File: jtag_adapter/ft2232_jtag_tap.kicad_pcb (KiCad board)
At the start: 2 copper layers, 50 x 30 mm, 50 parts, among them J1 USB_C_Receptacle_USB2.0, J2 Conn_ARM_JTAG_SWD_20, U1 93AA56BT-I/OT, U2 FT232HL, Y1 Crystal_GND24

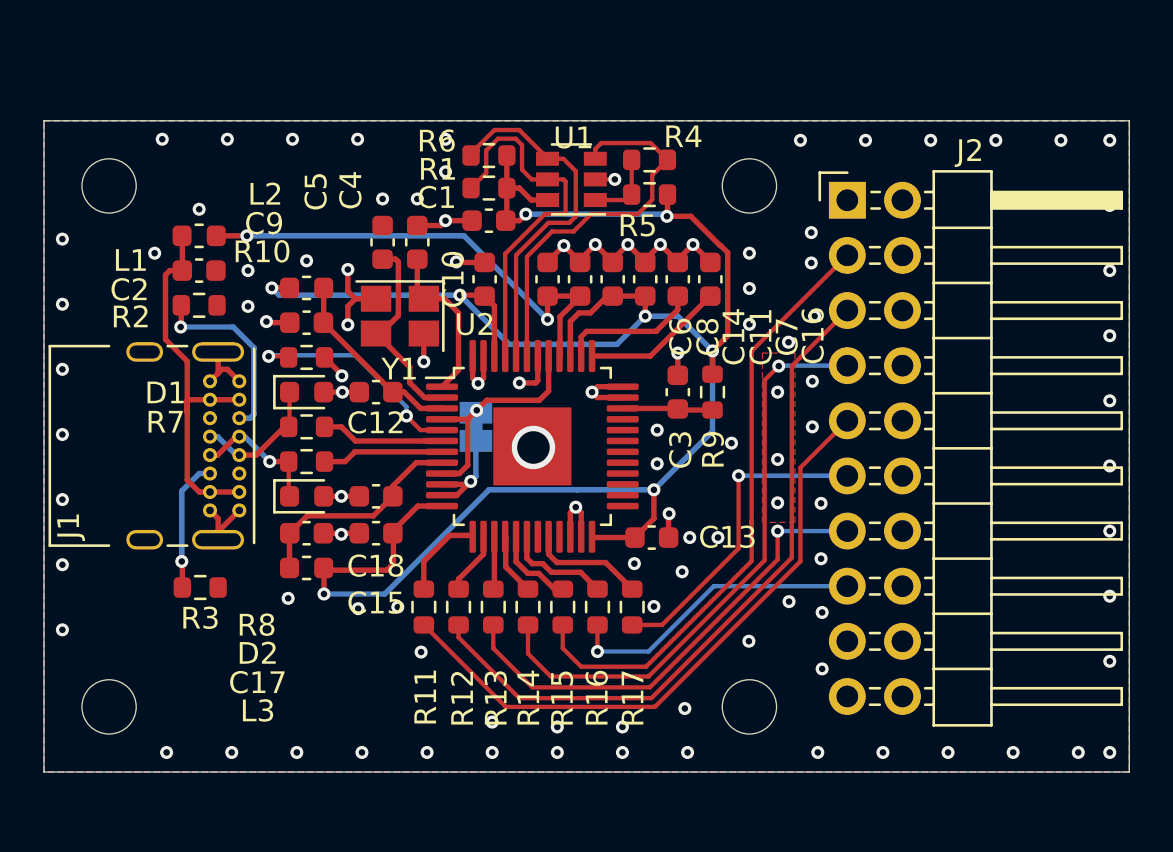
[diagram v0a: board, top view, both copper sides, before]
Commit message: v0.2に改修
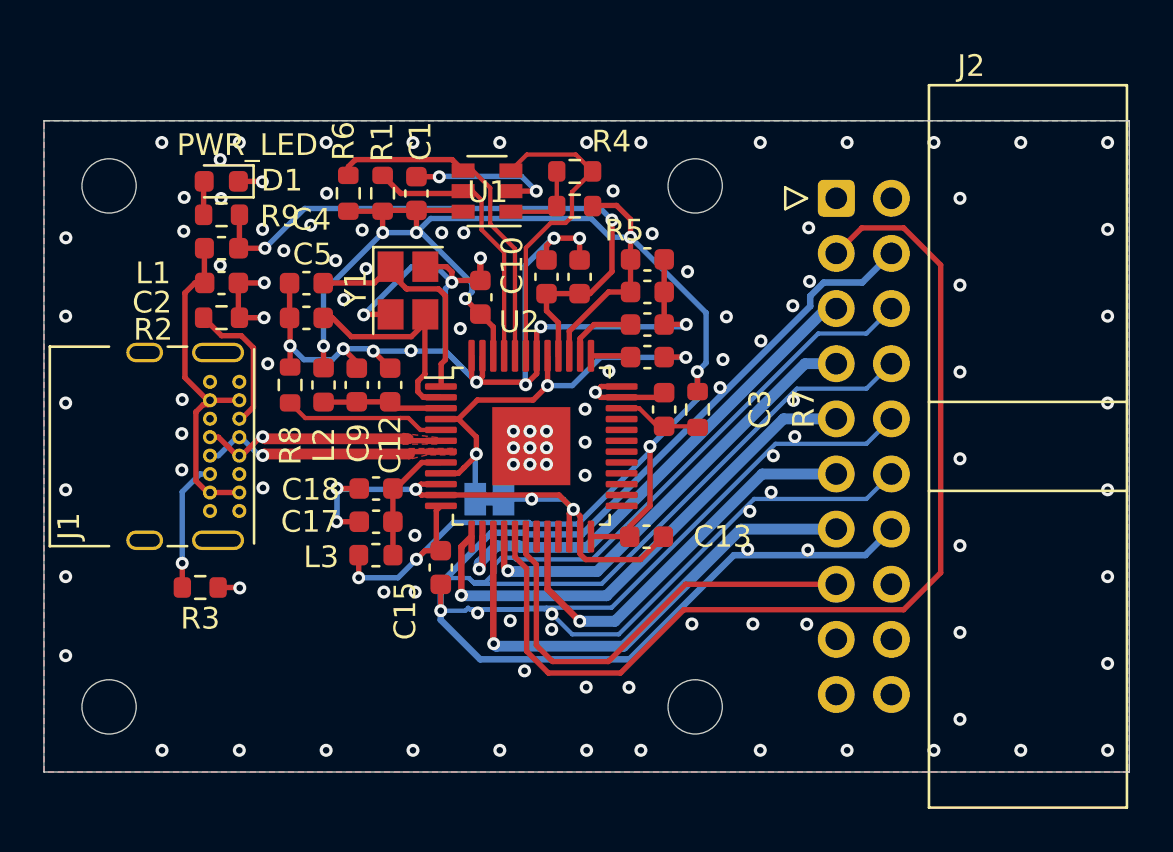
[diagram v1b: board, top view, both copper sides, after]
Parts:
- removed D2: PGB1010603, Diode_SMD:D_0603_1608Metric
- removed R10: 10k, Resistor_SMD:R_0603_1608Metric
- removed R11, R12, R13, R14, R15, R16, R17: 0, Resistor_SMD:R_0603_1608Metric
- D1: value PGB1010603 -> PWR_LED; footprint Diode_SMD:D_0603_1608Metric -> LED_SMD:LED_0603_1608Metric
- J2: footprint Connector_PinHeader_2.54mm:PinHeader_2x10_P2.54mm_Horizontal -> Connector_IDC:IDC-Header_2x10_P2.54mm_Horizontal
- R7: value 0 -> 10k
- R8: value 0 -> 12k/1%
- R9: value 10k -> 1k
- moved R9 24.1 mm to (58.2, 104.3), turned to 0 degrees
- moved R7 18.0 mm to (80.1, 113.3), turned to 90 degrees
- moved D1 10.5 mm to (58.2, 102.8), turned to 180 degrees
- moved R6 6.71 mm to (64.0, 103.3), turned to 270 degrees
- moved C4 5.44 mm to (62.1, 107.5), turned to 180 degrees
- moved C5 4.94 mm to (62.1, 109.1), turned to 180 degrees
- moved R1 4.90 mm to (65.6, 103.3), turned to 270 degrees
- moved C16 4.61 mm to (77.8, 110.9), turned to 0 degrees
- moved L2 4.54 mm to (62.9, 112.2), turned to 90 degrees
- moved U1 3.93 mm to (70.4, 103.2)
- moved C9 3.68 mm to (64.4, 112.2), turned to 90 degrees
- moved R8 3.61 mm to (61.3, 112.2), turned to 270 degrees
- moved C1 3.57 mm to (67.2, 103.3), turned to 90 degrees
- moved R4 3.49 mm to (74.5, 103.9)
- moved R5 3.49 mm to (74.5, 102.3)
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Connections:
- C16 pad 2: GND -> GNDA
- D1 pad 1: Net-(D1-Pad1) -> GND
- D1 pad 2: GND -> Net-(D1-Pad2)
- J1 pad A6: Net-(D2-Pad1) -> /USB_D+
- J1 pad A7: Net-(D1-Pad1) -> /USB_D-
- J1 pad B6: Net-(D2-Pad1) -> /USB_D+
- J1 pad B7: Net-(D1-Pad1) -> /USB_D-
- R7 pad 1: /USB_D- -> Net-(C3-Pad1)
- R7 pad 2: Net-(D1-Pad1) -> +3V3
- R8 pad 1: /USB_D+ -> GND
- R8 pad 2: Net-(D2-Pad1) -> Net-(R8-Pad2)
- R9 pad 1: Net-(C3-Pad1) -> Net-(D1-Pad2)
- R9 pad 2: +3V3 -> +5V
- U2 pad 13: Net-(R11-Pad2) -> /SK_TCK
- U2 pad 14: Net-(R12-Pad2) -> /DO_TDI
- U2 pad 15: Net-(R13-Pad2) -> /DI_TDO
- U2 pad 16: Net-(R14-Pad2) -> /CS_TMS
- U2 pad 17: Net-(R15-Pad2) -> /~SRST
- U2 pad 18: Net-(R16-Pad2) -> /~TRST
- U2 pad 20: Net-(R17-Pad2) -> /RTCK
- U2 pad 49: GND -> (no net)
- U2 pad 5: Net-(R10-Pad2) -> Net-(R8-Pad2)
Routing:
- net GND: track 52.3 -> 259.4 mm, vias 107 -> 124
- net /~SRST: track 28.2 -> 47.1 mm
- net Net-(R10-Pad2): track 10.6 -> 0.00 mm, vias 2 -> 0
- net GNDA: track 10.5 -> 21.0 mm, vias 1 -> 3
- net +3V3: track 95.0 -> 84.7 mm, vias 8 -> 9
- net /DO_TDI: track 32.2 -> 23.2 mm, vias 0 -> 1
- net Net-(R8-Pad2): track 0.00 -> 7.47 mm
- net /~TRST: track 14.0 -> 20.8 mm, vias 1 -> 0
- net /CS_TMS: track 27.3 -> 20.8 mm
- net +5V: track 22.6 -> 28.9 mm
- net Net-(D1-Pad1): track 6.13 -> 0.00 mm
- net Net-(D2-Pad1): track 6.07 -> 0.00 mm, vias 1 -> 0
- net /USB_D+: track 5.60 -> 11.4 mm, vias 0 -> 1
- net /USB_D-: track 5.68 -> 11.5 mm, vias 0 -> 1
- net /SK_TCK: track 29.1 -> 23.6 mm, vias 0 -> 1
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- added copper zone on F.Cu, net /USB_D+
- added copper zone on F.Cu, net /USB_D-
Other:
- board text added: "PWR_LED"
- board text added: "jtag adapter v0.2(2021.07.17) @tnishinaga"
- board text removed: "jtag adapter v0.1(2021.05.15) @tnishinaga"
